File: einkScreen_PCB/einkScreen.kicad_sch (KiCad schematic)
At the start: 75 parts, among them J1 GPIOS, J2 ICSP, J3 FH34SRJ-24S-0.5SH_50_, Q1 BSS138LT1G, Q2 BSS84LT1G, SW1 SW_Push, SW2 SW_Push, U1 ATmega328P-A, U2 ST25DV64K-JFR6D3, U3 TPS3839G25, U4 LD39050PUR, U5 TPS3839G33, Y2 X322516MOB4SI

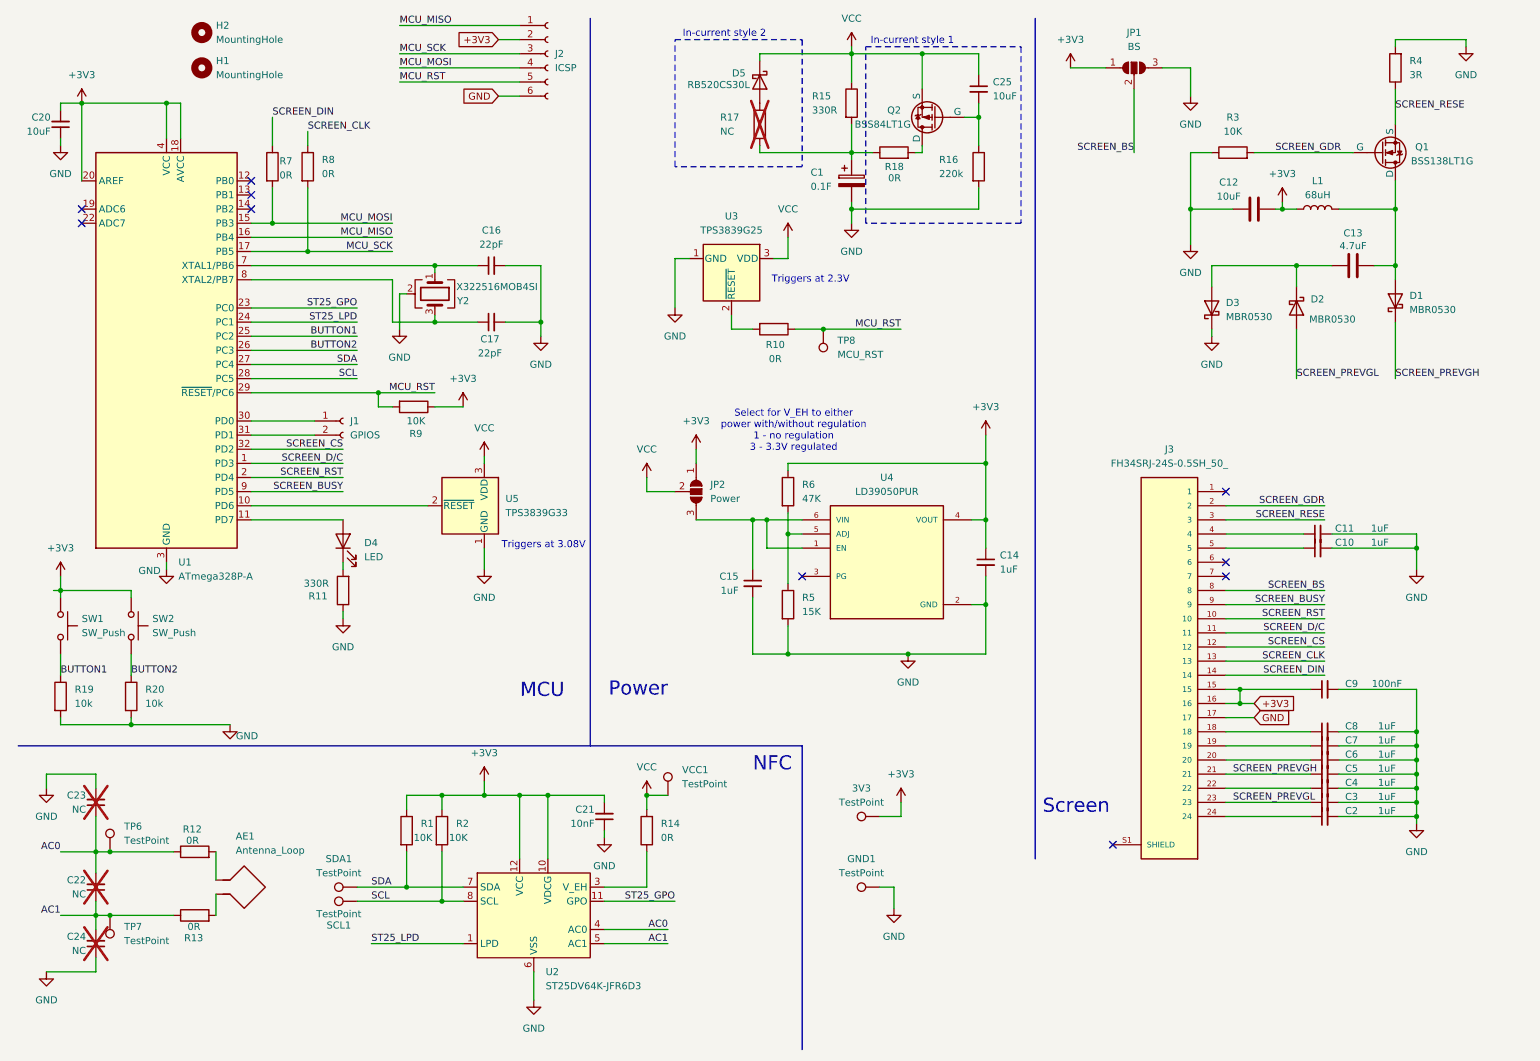
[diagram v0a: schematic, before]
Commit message: working BLE
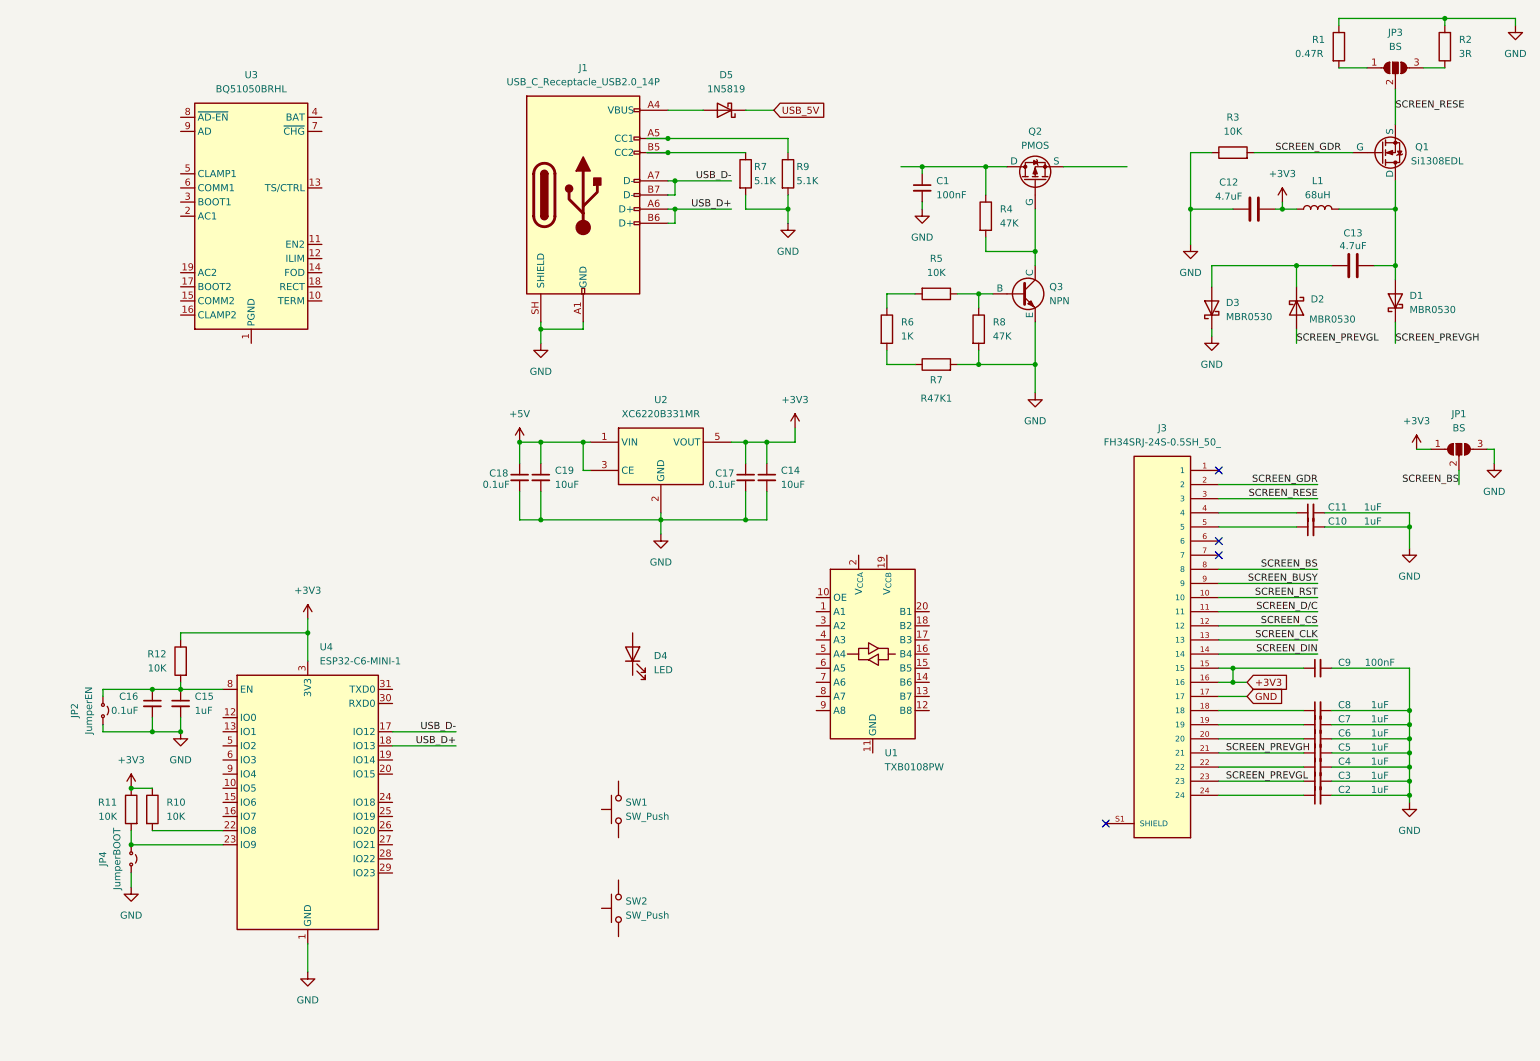
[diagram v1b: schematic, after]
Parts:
- removed 3V3, GND1, SCL1, SDA1, TP6, TP7, VCC1: TestPoint, TestPoint:TestPoint_Pad_2.5x2.5mm, symbol Connector:TestPoint
- removed AE1: Antenna_Loop, PCB Coils:COIL_GENERATOR, symbol Device:Antenna_Loop
- removed C1: 0.1F, Ironies_Libs:SuperCapacitor, symbol Device:C_Polarized
- removed C20, C25: 10uF, Capacitor_SMD:C_0805_2012Metric, symbol Device:C_Small
- removed C21: 10nF, Capacitor_SMD:C_0805_2012Metric, symbol Device:C_Small
- removed C22, C23, C24: NC, Capacitor_SMD:C_0805_2012Metric_Pad1.18x1.45mm_HandSolder, symbol Device:C_Small
- removed H1, H2: MountingHole, MountingHole:MountingHole_2.2mm_M2, symbol Mechanical:MountingHole
- removed J1: GPIOS, Connector_PinHeader_2.54mm:PinHeader_1x02_P2.54mm_Vertical, symbol Connector:Conn_01x02_Socket
- removed J2: ICSP, Connector_PinHeader_2.54mm:PinHeader_2x03_P2.54mm_Vertical, symbol Connector:Conn_01x06_Socket
- removed JP2: Power, Jumper:SolderJumper-3_P1.3mm_Open_RoundedPad1.0x1.5mm_NumberLabels, symbol Jumper:SolderJumper_3_Open
- removed R13, R14, R18: 0R, Resistor_SMD:R_0805_2012Metric_Pad1.20x1.40mm_HandSolder, symbol Device:R
- removed R15: 330R, Resistor_SMD:R_0805_2012Metric_Pad1.20x1.40mm_HandSolder, symbol Device:R
- removed R16: 220k, Resistor_SMD:R_0805_2012Metric, symbol Device:R
- removed R17: NC, Resistor_SMD:R_0805_2012Metric_Pad1.20x1.40mm_HandSolder, symbol Device:R
- removed R19, R20: 10k, Resistor_SMD:R_0805_2012Metric, symbol Device:R
- removed R2: 10K, Resistor_SMD:R_0805_2012Metric, symbol Device:R
- removed TP8: MCU_RST, TestPoint:TestPoint_Pad_2.5x2.5mm, symbol Connector:TestPoint
- removed U1: ATmega328P-A, Package_QFP:TQFP-32_7x7mm_P0.8mm, symbol MCU_Microchip_ATmega:ATmega328P-A
- removed U2: ST25DV64K-JFR6D3, Package_DFN_QFN:ST_UFDFPN-12-1EP_3x3mm_P0.5mm_EP1.4x2.55mm, symbol RF_NFC:ST25DV64K-JFR6D3
- removed U3: TPS3839G25, Package_TO_SOT_SMD:SOT-23, symbol Power_Supervisor:TPS3839DBZ
- removed U4: LD39050PUR, LD39050PUR:SON95P300X300X100-7N, symbol LD39050PUR:LD39050PUR
- removed U5: TPS3839G33, Package_TO_SOT_SMD:SOT-23, symbol Power_Supervisor:TPS3839DBZ
- removed Y2: X322516MOB4SI, Crystal:Crystal_SMD_SeikoEpson_TSX3225-4Pin_3.2x2.5mm, symbol Device:Crystal_GND24
- added C1: 100nF, symbol Device:C_Small
- added C18: 0.1uF, symbol Device:C_Small
- added C19: 10uF, symbol Device:C_Small
- added J1: USB_C_Receptacle_USB2.0_14P, symbol Connector:USB_C_Receptacle_USB2.0_14P
- added JP2: JumperEN, symbol Jumper:Jumper_2_Small_Open
- added JP3: BS, Jumper:SolderJumper-3_P1.3mm_Open_RoundedPad1.0x1.5mm_NumberLabels, symbol Jumper:SolderJumper_3_Open
- added JP4: JumperBOOT, symbol Jumper:Jumper_2_Small_Open
- added Q3: NPN, symbol Simulation_SPICE:NPN
- added R4: 47K, symbol Device:R
- added R47K1: R7, symbol Device:R
- added U1: TXB0108PW, Package_SO:TSSOP-20_4.4x6.5mm_P0.65mm, symbol Logic_LevelTranslator:TXB0108PW
- added U2: XC6220B331MR, Package_TO_SOT_SMD:SOT-23-5, symbol Regulator_Linear:XC6220B331MR
- added U3: BQ51050BRHL, Package_DFN_QFN:Texas_VQFN-RHL-20, symbol Battery_Management:BQ51050BRHL
- added U4: ESP32-C6-MINI-1, RF_Module:ESP32-C6-MINI-1, symbol RF_Module:ESP32-C6-MINI-1
- C12: value 10uF -> 4.7uF; LCSC C15850 -> (none)
- C14: value 1uF -> 10uF; footprint Capacitor_SMD:C_0805_2012Metric -> (none); LCSC C28323 -> (none)
- C15: footprint Capacitor_SMD:C_0805_2012Metric -> (none); LCSC C28323 -> (none)
- C16, C17: value 22pF -> 0.1uF; footprint Capacitor_SMD:C_0805_2012Metric -> (none); LCSC C1804 -> (none)
- D4: footprint LED_SMD:LED_0805_2012Metric -> (none); LCSC C2297 -> (none)
- D5: value RB520CS30L -> 1N5819; footprint Diode_SMD:D_SOD-882 -> (none); LCSC C2841401 -> (none)
- Q1: value BSS138LT1G -> Si1308EDL; LCSC C8490 -> (none)
- Q2: value BSS84LT1G -> PMOS; footprint Package_TO_SOT_SMD:SOT-23-3 -> (none); LCSC C8492 -> (none)
- R1: value 10K -> 0.47R; footprint Resistor_SMD:R_0805_2012Metric -> (none); LCSC C17414 -> (none)
- R10, R12: value 0R -> 10K; footprint Resistor_SMD:R_0805_2012Metric_Pad1.20x1.40mm_HandSolder -> (none); LCSC C17477 -> (none)
- R11: value 330R -> 10K; footprint Resistor_SMD:R_0805_2012Metric -> (none); LCSC C17630 -> (none)
- R5: value 15K -> 10K; footprint Resistor_SMD:R_0805_2012Metric -> (none); LCSC C17475 -> (none)
- R6: value 47K -> 1K; footprint Resistor_SMD:R_0805_2012Metric -> (none); LCSC C17713 -> (none)
- R7: value 0R -> 5.1K; footprint Resistor_SMD:R_0805_2012Metric_Pad1.20x1.40mm_HandSolder -> (none); LCSC C17477 -> (none)
- R8: value 0R -> 47K; footprint Resistor_SMD:R_0805_2012Metric_Pad1.20x1.40mm_HandSolder -> (none); LCSC C17477 -> (none)
- R9: value 10K -> 5.1K; footprint Resistor_SMD:R_0805_2012Metric -> (none); LCSC C17414 -> (none)
- SW1, SW2: footprint Button_Switch_SMD:Panasonic_EVQPUL_EVQPUC -> (none); LCSC C79174 -> (none)
- renumbered R4 to R2
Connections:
- net AC0 is gone; now on net +3V3: R12.1
- net MCU_MOSI is gone; now on net GND: R7.2
- net MCU_SCK is gone; now on net GND: R8.2
- net +3V3: now also C17.1, R10.1, R11.1, U2.5 (VOUT), U4.3 (3V3); no longer R1.1, R6.1, R9.1, SW1.1, SW2.1
- net GND: now also R1.1, R9.2, C1.2, C18.2, C19.2, J1.A1 (GND), J1.A12 (GND), J1.B1 (GND), J1.B12 (GND), J1.SH (SHIELD), JP2.2 (B), JP4.2 (B), Q3.3 (E), R47K1.2, U2.2 (GND), U4.1 (GND), U4.11 (GND), U4.14 (GND), U4.2 (GND), U4.36 (GND), U4.37 (GND), U4.38 (GND), U4.39 (GND), U4.40 (GND), U4.41 (GND), U4.42 (GND), U4.43 (GND), U4.44 (GND), U4.45 (GND), U4.46 (GND), U4.47 (GND), U4.48 (GND), U4.49 (GND), U4.50 (GND), U4.51 (GND), U4.52 (GND), U4.53 (GND); no longer R11.1, R5.2
- net SCREEN_CLK: no longer R8.1
- net SCREEN_DIN: no longer R7.1
- net SCREEN_RESE: now also JP3.2 (C); no longer R2.1
- net at C16.1: now also C15.1, R12.2, JP2.1 (A), U4.8 (EN)
- net at Q2.1 (D): now also C1.1, R4.1
- net at R6.2: now also R47K1.1; no longer R5.1
- net at R10.2: now also U4.22 (IO8)
- net at D5.2 (A): now also J1.A4 (VBUS), J1.A9 (VBUS), J1.B4 (VBUS), J1.B9 (VBUS)
- net at R11.2: now also JP4.1 (A), U4.23 (IO9); no longer D4.1 (K)
- net at Q2.2 (G): now also Q3.1 (C), R4.2
- net BUTTON1: no longer names the net of SW1.2
- net BUTTON2: no longer names the net of SW2.2
- removed net MCU_RST: R10.1, R9.2
- net SDA: no longer names the net of R1.2
- net SDA: now also JP3.1 (A)
- net VCC: no longer names the net of Q2.3 (S)
- net VCC: no longer D5.1 (K)
- new net: J1.A5 (CC1), R9.1
- new net: J1.B5 (CC2), R7.1
- new net: Q3.2 (B), R5.1, R8.1
- new net: JP3.3 (B), R2.1
- new net: R5.2, R6.1
- new net: U3.1 (PGND), U3.20 (PGND), U3.21 (PGND)
- new net +5V: C18.1, C19.1, U2.1 (VIN), U2.3 (CE)
- new net USB_5V: D5.1 (K)
- new net USB_D+: J1.A6 (D+), J1.B6 (D+), U4.18 (IO13)
- new net USB_D-: J1.A7 (D-), J1.B7 (D-), U4.17 (IO12)
- no-connect marks 10 -> 4
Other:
- note removed: "In-current style 1"
- note removed: "In-current style 2"
- note removed: "MCU"
- note removed: "NFC"
- note removed: "Power"
- note removed: "Screen"
- note removed: "Select for V_EH to either power with/without regulation 1 - no regulation 3 - 3.3V regulated"
- note removed: "Triggers at 2.3V"
- note removed: "Triggers at 3.08V"
- moved on the sheet: C10, C11, C2, C3, C4, C5, C6, C7, C8, C9, J3, JP1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

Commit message: working kinda
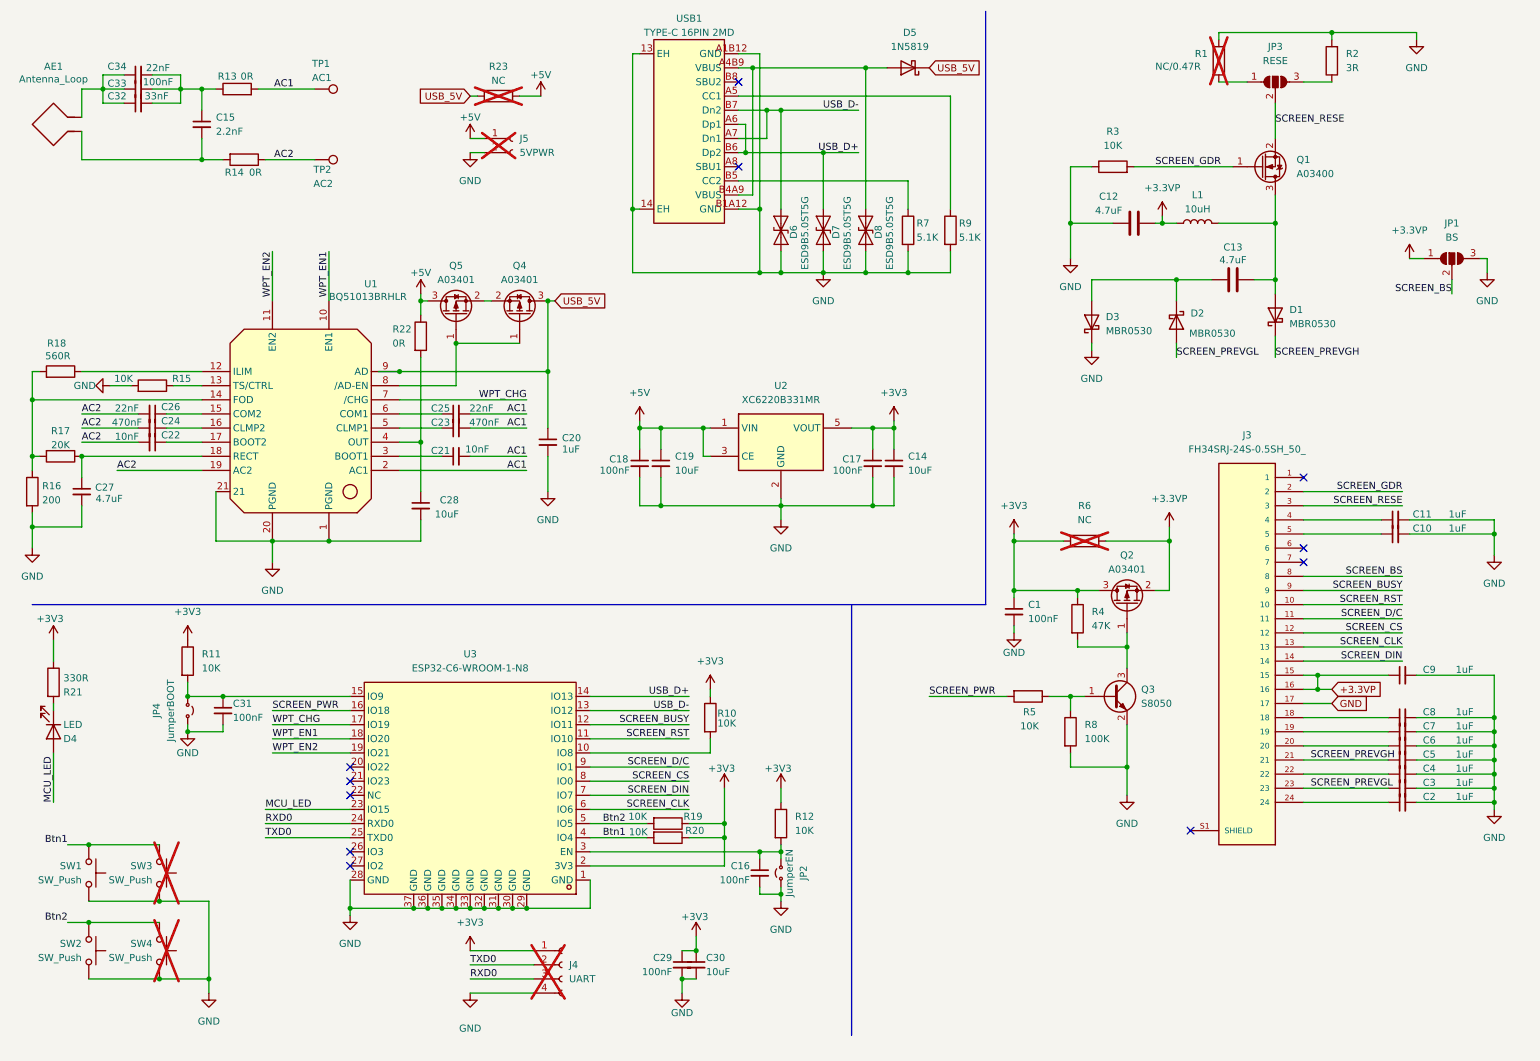
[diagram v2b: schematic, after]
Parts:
- removed J1: USB_C_Receptacle_USB2.0_14P, symbol Connector:USB_C_Receptacle_USB2.0_14P
- removed Q1: Si1308EDL, Package_TO_SOT_SMD:SOT-23-3, symbol Simulation_SPICE:NMOS
- removed Q2: PMOS, symbol Simulation_SPICE:PMOS
- removed Q3: NPN, symbol Simulation_SPICE:NPN
- removed R47K1: R7, symbol Device:R
- removed U1: TXB0108PW, Package_SO:TSSOP-20_4.4x6.5mm_P0.65mm, symbol Logic_LevelTranslator:TXB0108PW
- removed U3: BQ51050BRHL, Package_DFN_QFN:Texas_VQFN-RHL-20, symbol Battery_Management:BQ51050BRHL
- removed U4: ESP32-C6-MINI-1, RF_Module:ESP32-C6-MINI-1, symbol RF_Module:ESP32-C6-MINI-1
- added AE1: Antenna_Loop, PCB Coils:WPT_COIL, symbol Device:Antenna_Loop
- added C20: 1uF, Capacitor_SMD:C_0805_2012Metric, symbol Device:C_Small
- added C21, C22: 10nF, Capacitor_SMD:C_0805_2012Metric, symbol Device:C_Small
- added C23, C24: 470nF, Capacitor_SMD:C_0805_2012Metric, symbol Device:C_Small
- added C25, C26, C34: 22nF, Capacitor_SMD:C_0805_2012Metric, symbol Device:C_Small
- added C27: 4.7uF, Capacitor_SMD:C_0805_2012Metric, symbol Device:C_Small
- added C28, C30: 10uF, Capacitor_SMD:C_0805_2012Metric, symbol Device:C_Small
- added C29, C31, C33: 100nF, Capacitor_SMD:C_0805_2012Metric, symbol Device:C_Small
- added C32: 33nF, Capacitor_SMD:C_0805_2012Metric, symbol Device:C_Small
- added D6, D7, D8: ESD9B5.0ST5G, Diode_SMD:D_SOD-923, symbol Diode:ESD9B5.0ST5G
- added J4: UART, Connector_PinSocket_2.54mm:PinSocket_1x04_P2.54mm_Vertical, symbol Connector:Conn_01x04_Socket
- added J5: 5VPWR, Connector_PinSocket_2.54mm:PinSocket_1x02_P2.54mm_Vertical, symbol Connector:Conn_01x02_Socket
- added Q1: A03400, Package_TO_SOT_SMD:TSOT-23, symbol Transistor_FET_Other:Q_NMOS_Depletion_GSD
- added Q2, Q4, Q5: A03401, Package_TO_SOT_SMD:TSOT-23, symbol Transistor_FET:Q_PMOS_GSD
- added Q3: S8050, Package_TO_SOT_SMD:TSOT-23, symbol Transistor_BJT:Q_NPN_BEC
- added R13, R14, R22: 0R, Resistor_SMD:R_0805_2012Metric, symbol Device:R
- added R15, R19, R20: 10K, Resistor_SMD:R_0805_2012Metric, symbol Device:R
- added R16: 200, Resistor_SMD:R_0805_2012Metric, symbol Device:R
- added R17: 20K, Resistor_SMD:R_0805_2012Metric, symbol Device:R
- added R18: 560R, Resistor_SMD:R_0805_2012Metric, symbol Device:R
- added R21: 330R, Resistor_SMD:R_0805_2012Metric, symbol Device:R
- added R23: NC, Resistor_SMD:R_0805_2012Metric, symbol Device:R
- added SW3, SW4: SW_Push, CustomButtons:KEY-SMD_L4.0-W3.0-LS4.9-1, symbol Switch:SW_Push
- added TP1: AC1, TestPoint:TestPoint_Pad_D3.0mm, symbol Connector:TestPoint
- added TP2: AC2, TestPoint:TestPoint_Pad_D3.0mm, symbol Connector:TestPoint
- added U1: BQ51013BRHLR, lcscDownloadLib:VQFN-20_L4.5-W3.5-P0.50-BL-EP_BQ24100RHLR, symbol lcscDownloadLib:BQ51013BRHLR
- added U3: ESP32-C6-WROOM-1-N8, lcscDownloadLib:WIRELM-SMD_ESP32-C6-WROOM-1, symbol lcscDownloadLib:ESP32-C6-WROOM-1-N8
- added USB1: TYPE-C 16PIN 2MD, lcscDownloadLib:USB-C-SMD_TYPE-C-16PIN-2MD-073, symbol easyeda2kicad:TYPE-C16PIN2MD
- C1: footprint (none) -> Capacitor_SMD:C_0805_2012Metric; LCSC (none) -> C28233
- C12: LCSC (none) -> C1779
- C14, C19: footprint (none) -> Capacitor_SMD:C_0805_2012Metric; LCSC (none) -> C15850
- C15: value 1uF -> 2.2nF; footprint (none) -> Capacitor_SMD:C_0805_2012Metric; LCSC (none) -> C28260
- C16, C17, C18: value 0.1uF -> 100nF; footprint (none) -> Capacitor_SMD:C_0805_2012Metric; LCSC (none) -> C28233
- C9: value 100nF -> 1uF; LCSC C28233 -> C28323
- D4: footprint (none) -> LED_SMD:LED_0805_2012Metric; LCSC (none) -> C84256
- D5: footprint (none) -> Diode_SMD:D_SOD-123; LCSC (none) -> C82544
- JP2, JP4: footprint (none) -> TestPoint:TestPoint_2Pads_Pitch2.54mm_Drill0.8mm
- JP3: value BS -> RESE
- L1: value 68uH -> 10uH
- R1: value 0.47R -> NC/0.47R; footprint (none) -> Resistor_SMD:R_0805_2012Metric; now not fitted
- R10, R11, R12, R5: footprint (none) -> Resistor_SMD:R_0805_2012Metric; LCSC (none) -> C17414
- R4: footprint (none) -> Resistor_SMD:R_0805_2012Metric; LCSC (none) -> C17713
- R6: value 1K -> NC; footprint (none) -> Resistor_SMD:R_0805_2012Metric; now not fitted
- R7, R9: footprint (none) -> Resistor_SMD:R_0805_2012Metric; LCSC (none) -> C27834
- R8: value 47K -> 100K; footprint (none) -> Resistor_SMD:R_0805_2012Metric; LCSC (none) -> C149504
- SW1, SW2: footprint (none) -> Button_Switch_SMD:Panasonic_EVQPUL_EVQPUC; LCSC (none) -> C79174
- U2: LCSC (none) -> C22466451
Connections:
- net +3V3: now also C1.1, R4.1, R6.1, C29.1, C30.1, J4.1 (Pin_1), Q2.3 (D), R19.1, R20.1, R21.1, U3.2 (3V3); no longer C12.2, C9.1, J3.15, J3.16, JP1.1 (A), L1.1
- net +5V: now also J5.1 (Pin_1), Q5.3 (D), R22.1, R23.2
- net GND: now also SW1.1, SW2.1, C20.2, C27.2, C28.2, C29.2, C30.2, C31.2, D6.1 (A1), D7.1 (A1), D8.1 (A1), J4.4 (Pin_4), J5.2 (Pin_2), Q3.2 (E), R15.2, R16.2, SW3.1, SW4.1, U1.1 (PGND), U1.20 (PGND), U1.21, U3.1 (GND), U3.28 (GND), U3.29 (GND), U3.30 (GND), U3.31 (GND), U3.32 (GND), U3.33 (GND), U3.34 (GND), U3.35 (GND), U3.36 (GND), U3.37 (GND), USB1.13 (EH), USB1.14 (EH), USB1.A1B12 (GND), USB1.B1A12 (GND); no longer C15.2
- net SCREEN_BUSY: now also U3.12 (IO11)
- net SCREEN_CLK: now also U3.6 (IO6)
- net SCREEN_CS: now also U3.8 (IO0)
- net SCREEN_DIN: now also U3.7 (IO7)
- net SCREEN_D/C: now also U3.9 (IO1)
- net SCREEN_GDR: now also Q1.1 (G)
- net SCREEN_RESE: now also Q1.2 (S)
- net SCREEN_RST: now also U3.11 (IO10)
- net USB_5V: now also C20.1, Q4.3 (D), R23.1, U1.9 (AD)
- net USB_D+: now also D7.2 (A2), U3.14 (IO13), USB1.A6 (Dp1), USB1.B6 (Dp2)
- net USB_D-: now also D6.2 (A2), U3.13 (IO12), USB1.A7 (Dn1), USB1.B7 (Dn2)
- net Btn2: now reaches SW2.2
- net Btn2: now also R19.2, SW4.2, U3.5 (IO5)
- net at R10.2: now also U3.10 (IO8)
- net at C16.1, JP2.1 (A), R12.2: now also U3.3 (EN); no longer C15.1
- net at R9.1: now also USB1.A5 (CC1)
- net +3.3VP: now reaches R6.2
- net +3.3VP: now also C12.2, C9.1, J3.15, J3.16, JP1.1 (A), L1.1, Q2.2 (S)
- net at R4.2: now also Q2.1 (G), Q3.3 (C)
- net at C13.2, D1.2 (A), L1.2: now also Q1.3 (D)
- net at D5.2 (A): now also D8.2 (A2), USB1.A4B9 (VBUS), USB1.B4A9 (VBUS)
- net at R7.1: now also USB1.B5 (CC2)
- net at R5.1, R8.1: now also Q3.1 (B)
- net at JP4.1 (A), R11.2: now also C31.1, U3.15 (IO9)
- net Btn1: now reaches SW1.2
- net Btn1: now also R20.2, SW3.2, U3.4 (IO4)
- net SCREEN_PWR: now reaches R5.2
- net SCREEN_PWR: now also U3.16 (IO18); no longer R6.1
- net at D4.1 (K): now also R21.2
- net MCU_LED: now reaches D4.2 (A)
- net MCU_LED: now also U3.23 (IO15)
- new net: AE1.1, C15.2, R14.2
- new net: AE1.2, C32.1, C33.1, C34.1
- new net: C24.1, U1.16 (CLMP2)
- new net: C25.1, U1.6 (COM1)
- new net: R16.1, R17.2, R18.2, U1.14 (FOD)
- new net: C23.1, U1.5 (CLMP1)
- new net: C22.1, U1.17 (BOOT2)
- new net: C28.1, R22.2, U1.4 (OUT)
- new net: C27.1, R17.1, U1.18 (RECT)
- new net: Q4.1 (G), Q5.1 (G), U1.8 (/AD-EN)
- new net: Q4.2 (S), Q5.2 (S)
- new net: R18.1, U1.12 (ILIM)
- new net: C15.1, C32.2, C33.2, C34.2, R13.1
- new net: C26.1, U1.15 (COM2)
- new net: C21.1, U1.3 (BOOT1)
- new net: R15.1, U1.13 (TS/CTRL)
- new net AC1: C21.2, C23.2, C25.2, R13.2, TP1.1, U1.2 (AC1)
- new net AC2: C22.2, C24.2, C26.2, R14.1, TP2.1, U1.19 (AC2)
- new net RXD0: J4.3 (Pin_3), U3.24 (RXD0)
- new net TXD0: J4.2 (Pin_2), U3.25 (TXD0)
- new net WPT_CHG: U1.7 (/CHG), U3.17 (IO19)
- new net WPT_EN1: U1.10 (EN1), U3.18 (IO20)
- new net WPT_EN2: U1.11 (EN2), U3.19 (IO21)
- no-connect marks 4 -> 11
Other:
- moved on the sheet: C1, C10, C11, C12, C13, C14, C16, C17, C18, C19, C2, C3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
